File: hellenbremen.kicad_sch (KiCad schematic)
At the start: 10 parts

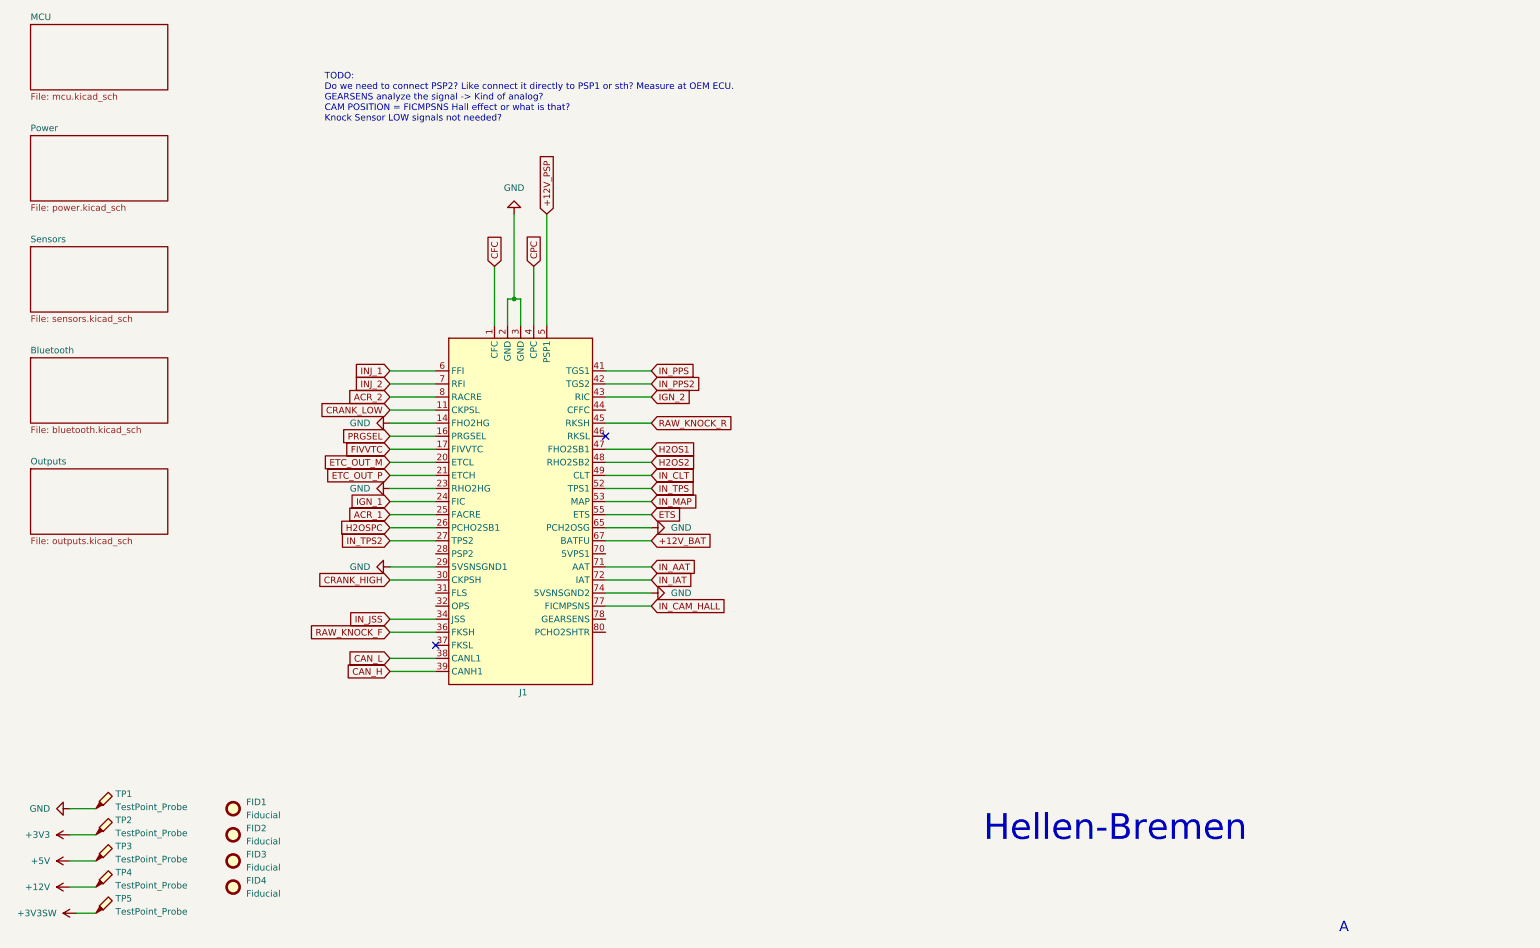
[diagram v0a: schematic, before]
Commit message: redone layout, possibly feature complete
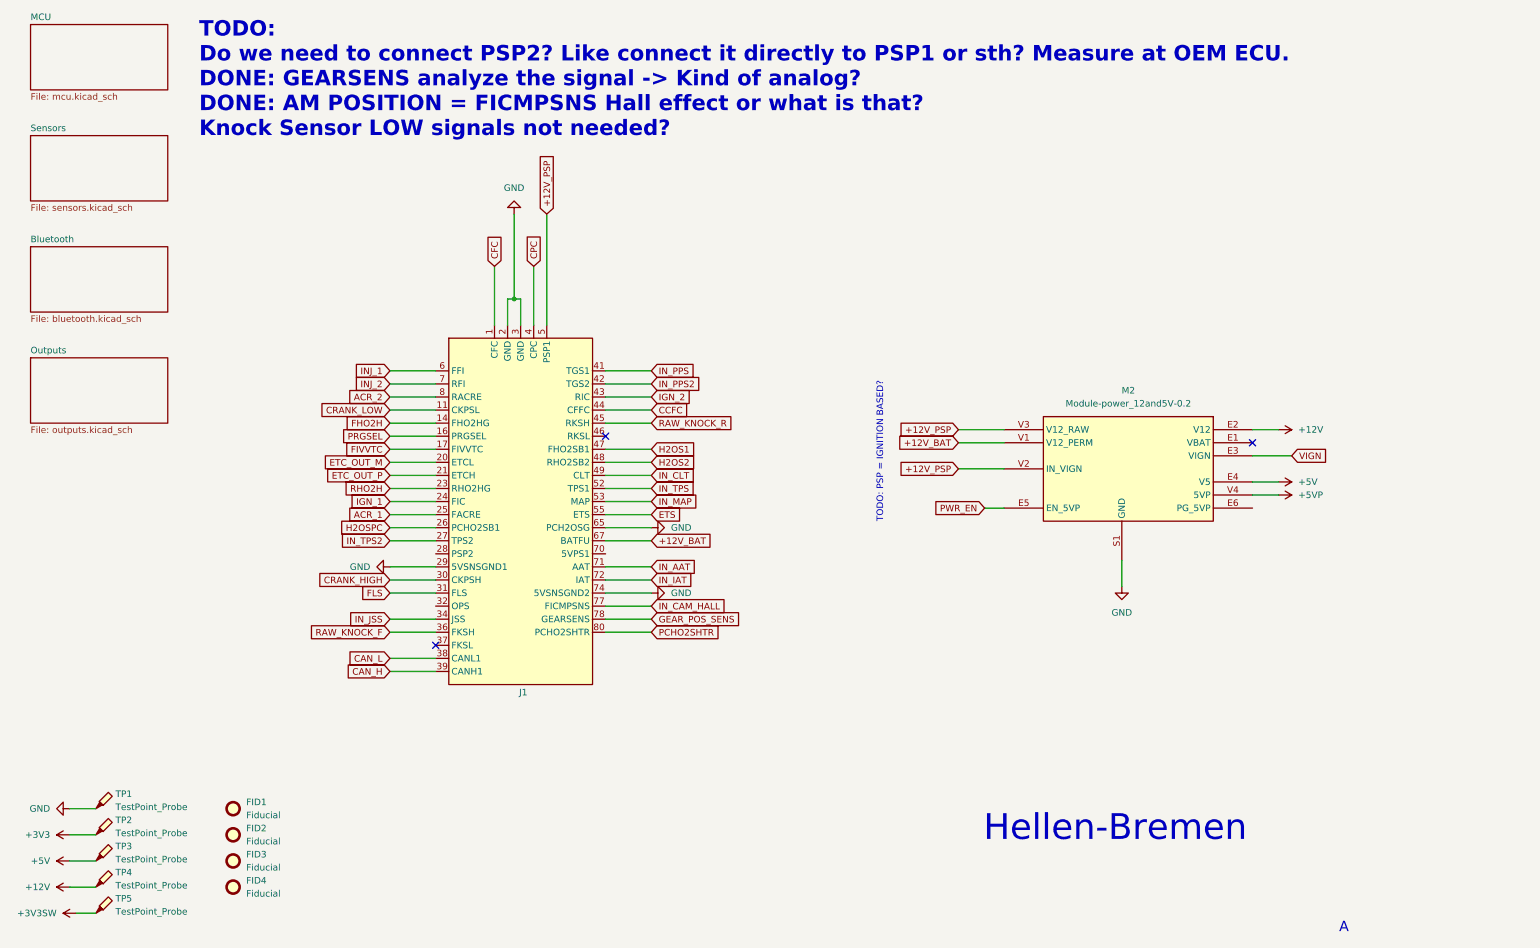
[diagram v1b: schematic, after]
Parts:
- added M2: Module-power_12and5V-0.2, 0.2:power_12and5V, symbol power_12and5V:Module-power_12and5V-0.2
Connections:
- net +12V: now also M2.E2 (V12)
- net +12V_BAT: now also M2.V1 (V12_PERM)
- net +12V_PSP: now also M2.V2 (IN_VIGN), M2.V3 (V12_RAW)
- net +5V: now also M2.E4 (V5)
- net GND: now also M2.S1 (GND); no longer J1.14 (FHO2HG), J1.23 (RHO2HG)
- net FLS: now reaches J1.31 (FLS)
- net CCFC: now reaches J1.44 (CFFC)
- net GEAR_POS_SENS: now reaches J1.78 (GEARSENS)
- net PCHO2SHTR: now reaches J1.80 (PCHO2SHTR)
- new net +5VP: M2.V4 (5VP)
- new net FHO2H: J1.14 (FHO2HG)
- new net PWR_EN: M2.E5 (EN_5VP)
- new net RHO2H: J1.23 (RHO2HG)
- new net VIGN: M2.E3 (VIGN)
- no-connect marks 2 -> 3
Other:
- removed sheet Power
- note added: "TODO: Do we need to connect PSP2? Like connect it directly to PSP1 or sth? Measure at OEM ECU. DONE: GEARSENS analyze the signal -> Kind of analog? DONE: AM POSITION = FICMPSNS Hall effect or what is that? Knock Sensor LOW signals not needed?"
- note added: "TODO: PSP = IGNITION BASED?"
- note removed: "TODO: Do we need to connect PSP2? Like connect it directly to PSP1 or sth? Measure at OEM ECU. GEARSENS analyze the signal -> Kind of analog? CAM POSITION = FICMPSNS Hall effect or what is that? Knock Sensor LOW signals not needed?"
